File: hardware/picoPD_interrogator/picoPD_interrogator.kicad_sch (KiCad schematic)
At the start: 53 parts, among them J1 Conn_01x07, J2 USB_C_Receptacle_USB2.0_16P, J3 Conn_01x14, Q1 rohm-RE1C002UN, Q2 rohm-RE1C002UN, Q3 rohm-RE1C002UN, Q4 rohm-RE1C002UN, Q5 rohm-RE1C002UN, SW1 RESET_BTN, U3 ST-LM393QT, U6 LV2862XDDC

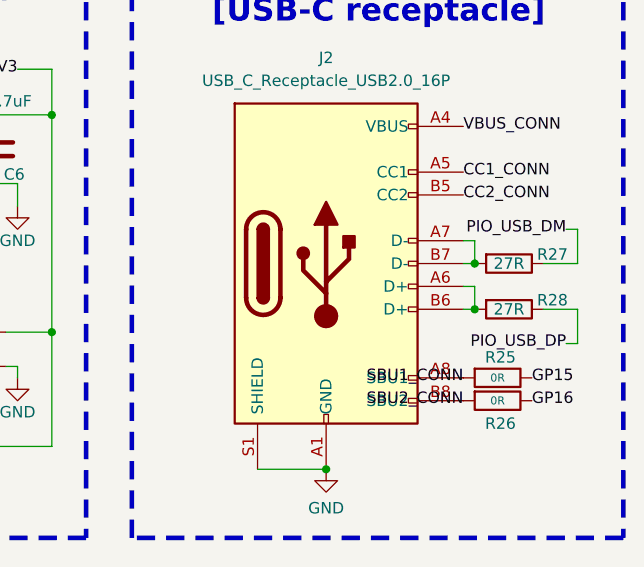
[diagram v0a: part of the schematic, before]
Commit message: PCB: Working on PCB layout.
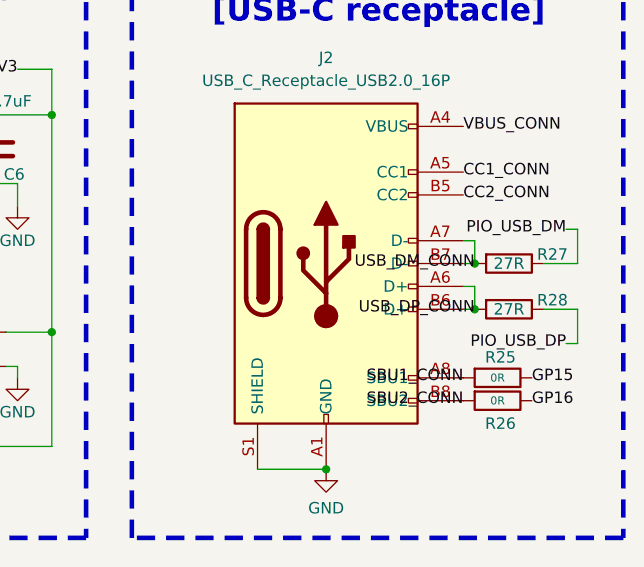
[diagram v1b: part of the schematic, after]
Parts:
- TP1: footprint TestPoint:TestPoint_Pad_D4.0mm -> TestPoint:TestPoint_Pad_D2.5mm
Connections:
- net USB_DM_CONN: now reaches J2.A7 (D-), J2.B7 (D-), R27.2
- net USB_DP_CONN: now reaches J2.A6 (D+), J2.B6 (D+), R28.2
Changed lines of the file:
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@@
 		)
 	)
+	(label "USB_DP_CONN"
+		(at 264.16 57.15 180)
+		(effects
+			(font
+				(size 1.27 1.27)
+			)
+			(justify right)
+		)
+	)
 	(label "CC2_TX_L"
 		(at 133.35 63.5 180)
@@
 		)
 	)
+	(label "USB_DM_CONN"
+		(at 264.16 52.07 180)
+		(effects
+			(font
+				(size 1.27 1.27)
+			)
+			(justify right)
+		)
+	)
 	(label "SCL"
 		(at 36.83 99.06 0)
@@
 			)
 		)
-		(property "Footprint" "TestPoint:TestPoint_Pad_D4.0mm"
+		(property "Footprint" "TestPoint:TestPoint_Pad_D2.5mm"
 			(at 156.21 179.07 0)
 			(effects

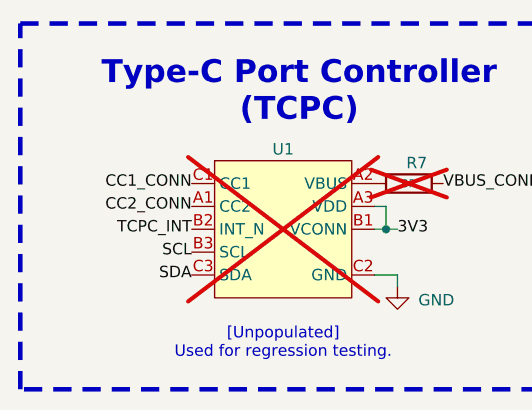
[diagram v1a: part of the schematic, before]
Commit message: PCB: Working on board layout.
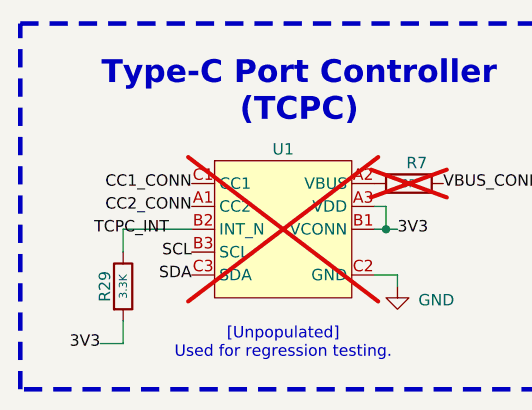
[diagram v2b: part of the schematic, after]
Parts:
- added R29: 3.3K, Resistor_SMD:R_0201_0603Metric, symbol Device:R
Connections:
- net 3V3: now also R29.2
- net TCPC_INT: now also R29.1
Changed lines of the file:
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@@
+	(wire
+		(pts
+			(xy 27.94 187.96) (xy 27.94 185.42)
+		)
+		(stroke
+			(width 0)
+			(type default)
+		)
+	)
 	(wire
 		(pts
@@
 	(wire
 		(pts
+			(xy 25.4 187.96) (xy 27.94 187.96)
+		)
+		(stroke
+			(width 0)
+			(type default)
+		)
+	)
+	(wire
+		(pts
+			(xy 27.94 177.8) (xy 27.94 175.26)
+		)
+		(stroke
+			(width 0)
+			(type default)
+		)
+	)
+	(wire
+		(pts
 			(xy 34.29 128.27) (xy 33.02 128.27)
 		)
@@
 		(pts
 			(xy 264.16 111.76) (xy 270.51 111.76)
+		)
+		(stroke
+			(width 0)
+			(type default)
+		)
+	)
+	(wire
+		(pts
+			(xy 27.94 175.26) (xy 35.56 175.26)
 		)
 		(stroke
@@
 	)
 	(label "TCPC_INT"
-		(at 35.56 175.26 180)
+		(at 33.02 175.26 180)
 		(effects
 			(font
@@
 			)
 			(justify left)
+		)
+	)
+	(label "3V3"
+		(at 25.4 187.96 180)
+		(effects
+			(font
+				(size 1.27 1.27)
+			)
+			(justify right)
 		)
 	)
@@
 					(unit 1)
 				)
+			)
+		)
+	)
+	(symbol
+		(lib_id "Device:R")
+		(at 27.94 181.61 0)
+		(unit 1)
+		(exclude_from_sim no)
+		(in_bom yes)
+		(on_board yes)
+		(dnp no)
+		(property "Reference" "R29"
+			(at 25.908 181.61 90)
+			(effects
+				(font
+					(size 1.27 1.27)
+				)
+			)
+		)
+		(property "Value" "3.3K"
+			(at 27.94 181.61 90)
+			(effects
+				(font
+					(size 0.889 0.889)
+				)
+			)
+		)
+		(property "Footprint" "Resistor_SMD:R_0201_0603Metric"
+			(at 26.162 181.61 90)
+			(effects
+				(font
+					(size 1.27 1.27)
+				)
+				(hide yes)
+			)
+		)
+		(property "Datasheet" "~"
+			(at 27.94 181.61 0)
+			(effects
+				(font
+					(size 1.27 1.27)
+				)
+				(hide yes)
+			)
+		)
+		(property "Description" "Resistor"
+			(at 27.94 181.61 0)
+			(effects
+				(font
+					(size 1.27 1.27)
+				)
+				(hide yes)
+			)
+		)
+		(property "Manufacturer" "Panasonic Electronic Components"
+			(at 27.94 181.61 0)
+			(effects
+				(font
+					(size 1.27 1.27)
+				)
+				(hide yes)
+			)
+		)
+		(property "Description Detailed" "3.3 kOhms ±1% 0.05W, 1/20W Chip Resistor 0201 (0603 Metric) Thick Film"
+			(at 27.94 181.61 0)
+			(effects
+				(font
+					(size 1.27 1.27)
+				)
+				(hide yes)
+			)
+		)
+		(property "DigiKey PN" "P122937CT-ND"
+			(at 27.94 181.61 0)
+			(effects
+				(font
+					(size 1.27 1.27)
+				)
+				(hide yes)
+			)
+		)
+		(property "Manufacturer PN" "ERJ-1GNF3301C"
+			(at 27.94 181.61 0)
+			(effects
+				(font
+					(size 1.27 1.27)
+				)
+				(hide yes)
+			)
+		)
+		(pin "1"
+		)
+		(pin "2"
+		)
+		(instances
+			(project "picoPD_interrogator"
+				(path "/e34b0978-7def-4921-94d0-accc0a677529"
+					(reference "R29")
+					(unit 1)
+				)
